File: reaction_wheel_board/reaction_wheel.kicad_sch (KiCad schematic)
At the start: 18 parts, among them U1 DRV8317HREER

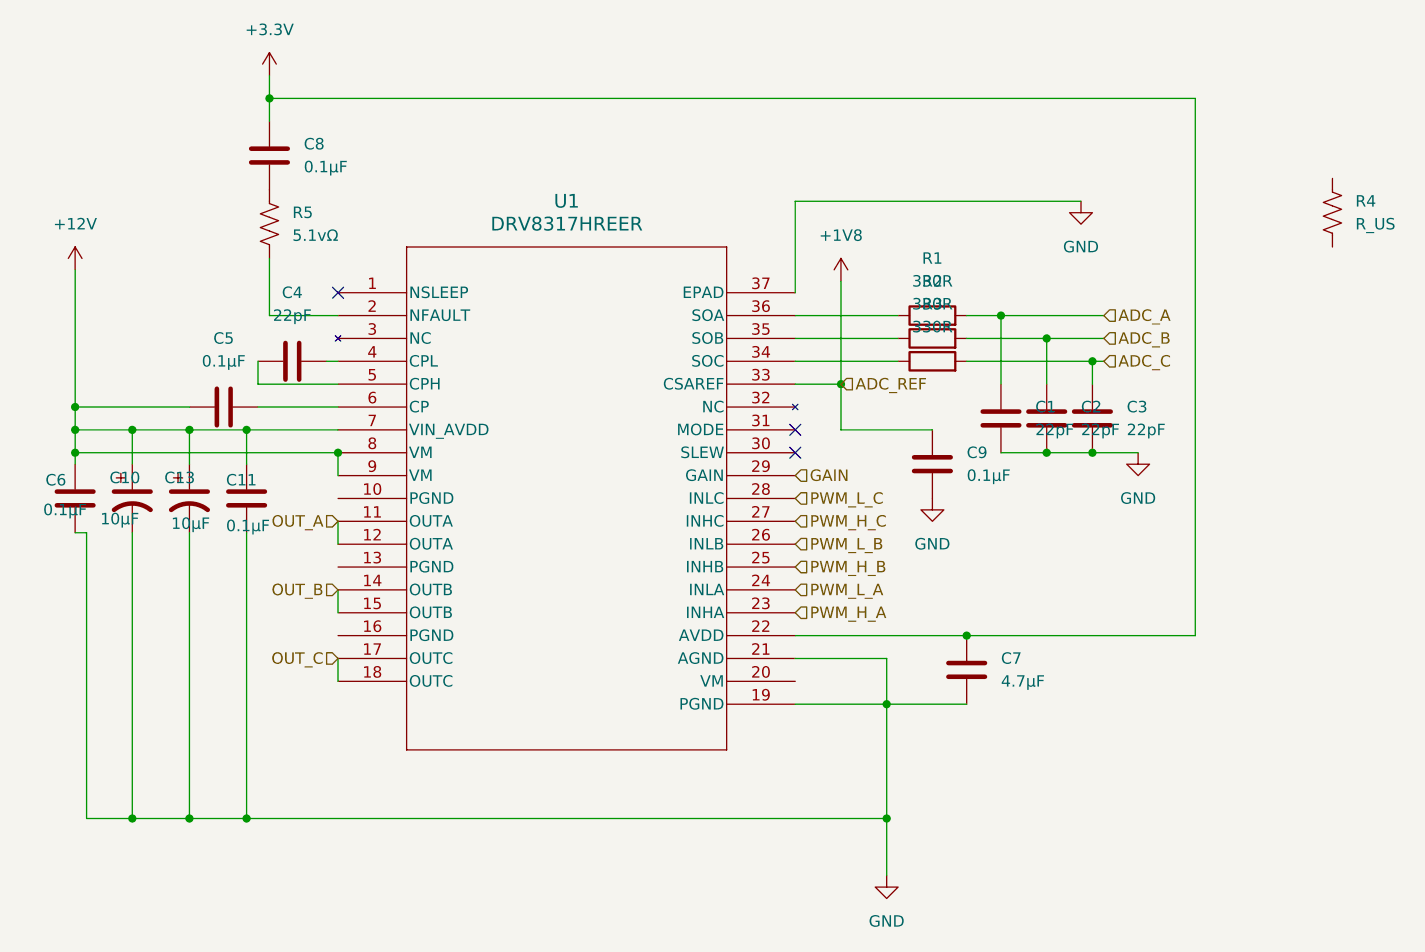
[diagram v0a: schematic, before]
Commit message: pcb layouts
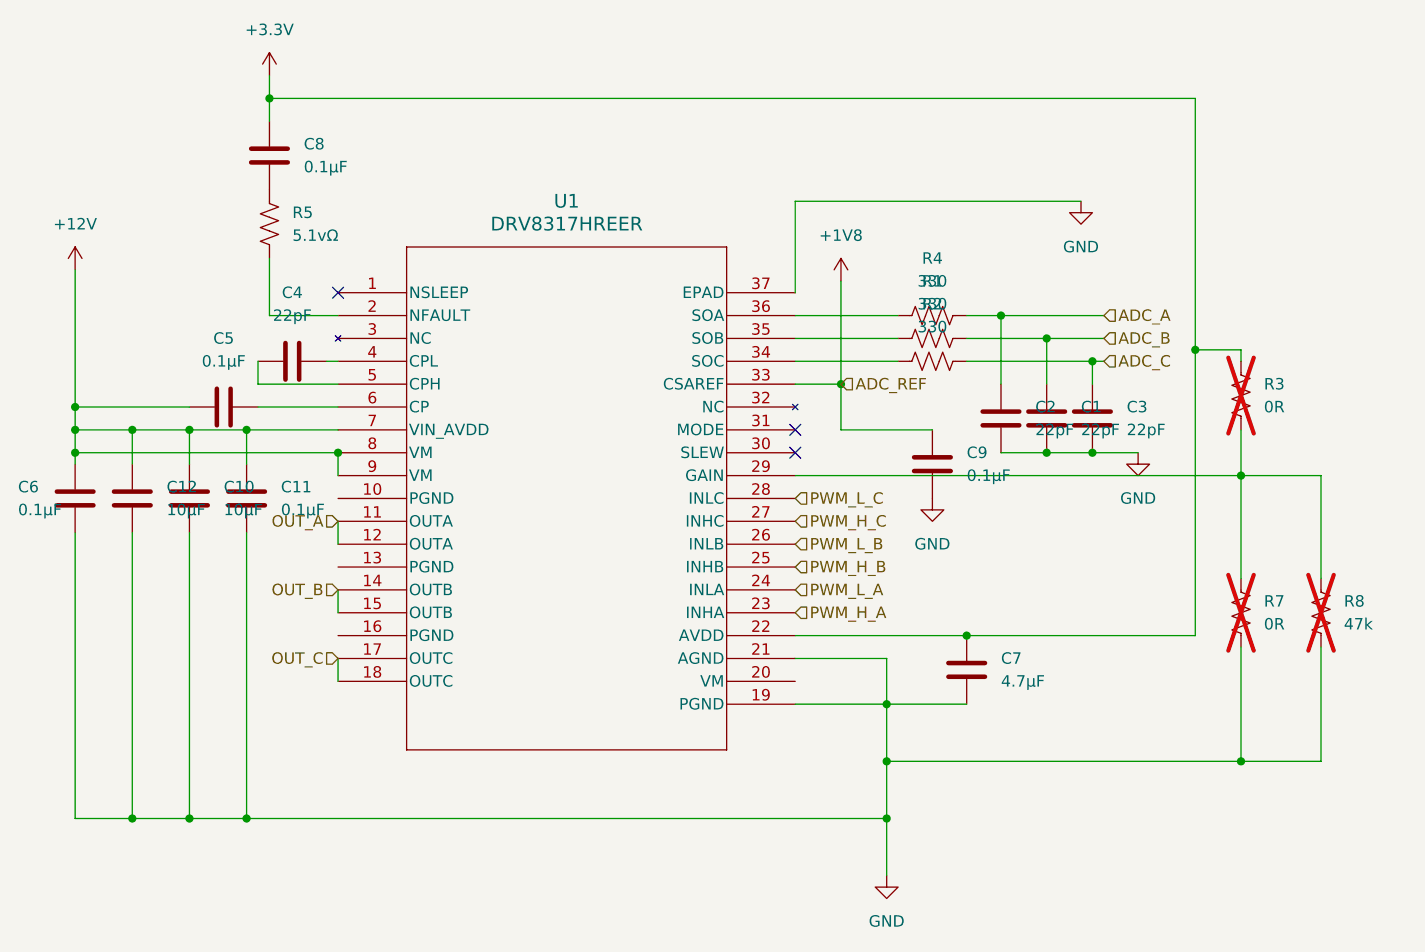
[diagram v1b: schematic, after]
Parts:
- removed C10, C13: 10μF, symbol Device:C_Polarized_US
- removed R1, R2, R3: 330R, symbol Device:R
- added C10, C12: 10μF, Capacitor_SMD:C_0603_1608Metric, symbol Device:C
- added R1, R2: 330, Resistor_SMD:R_0603_1608Metric, symbol Device:R_US
- added R3, R7: 0R, Resistor_SMD:R_0603_1608Metric, symbol Device:R_US
- added R8: 47k, Resistor_SMD:R_0603_1608Metric, symbol Device:R_US
- C1, C11, C2, C3, C4, C5, C6, C7, C8, C9: footprint (none) -> Capacitor_SMD:C_0603_1608Metric
- R4: value R_US -> 330; footprint (none) -> Resistor_SMD:R_0603_1608Metric
- R5: footprint (none) -> Resistor_SMD:R_0603_1608Metric
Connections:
- net +12V: now also C11.2, C6.2, C10.2, C12.2; no longer C11.1, C6.1
- net +3.3V: now also R3.2
- net ADC_A: now also C2.1, R4.2; no longer C1.1
- net ADC_B: now also C1.1, R1.2; no longer C2.1
- net ADC_C: now also R2.2
- net GND: now also C11.1, C6.1, C10.1, C12.1, R7.1, R8.1; no longer C11.2, C6.2
- net at R4.1: now also U1.36 (SOA)
- net at U1.34 (SOC): now also R2.1
- net at U1.35 (SOB): now also R1.1
- net GAIN: no longer names the net of U1.29 (GAIN)
- net GAIN: now also R3.1, R7.2, R8.2
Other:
- moved on the sheet: R4
